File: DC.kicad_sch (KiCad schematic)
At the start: 39 parts, among them U6 MCP2551-I-P, U7 NUCLEO-F302R8

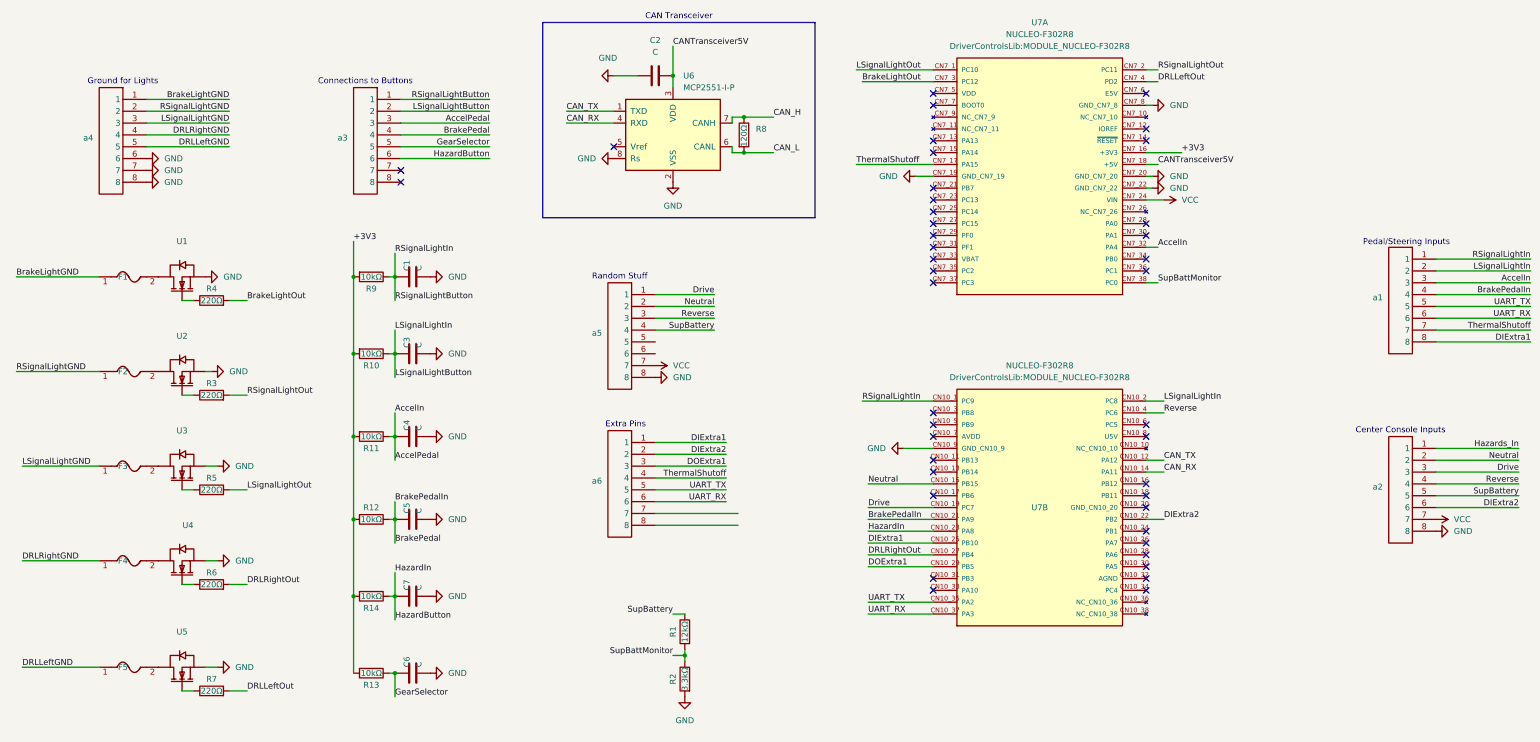
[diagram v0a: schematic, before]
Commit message: almost final draft
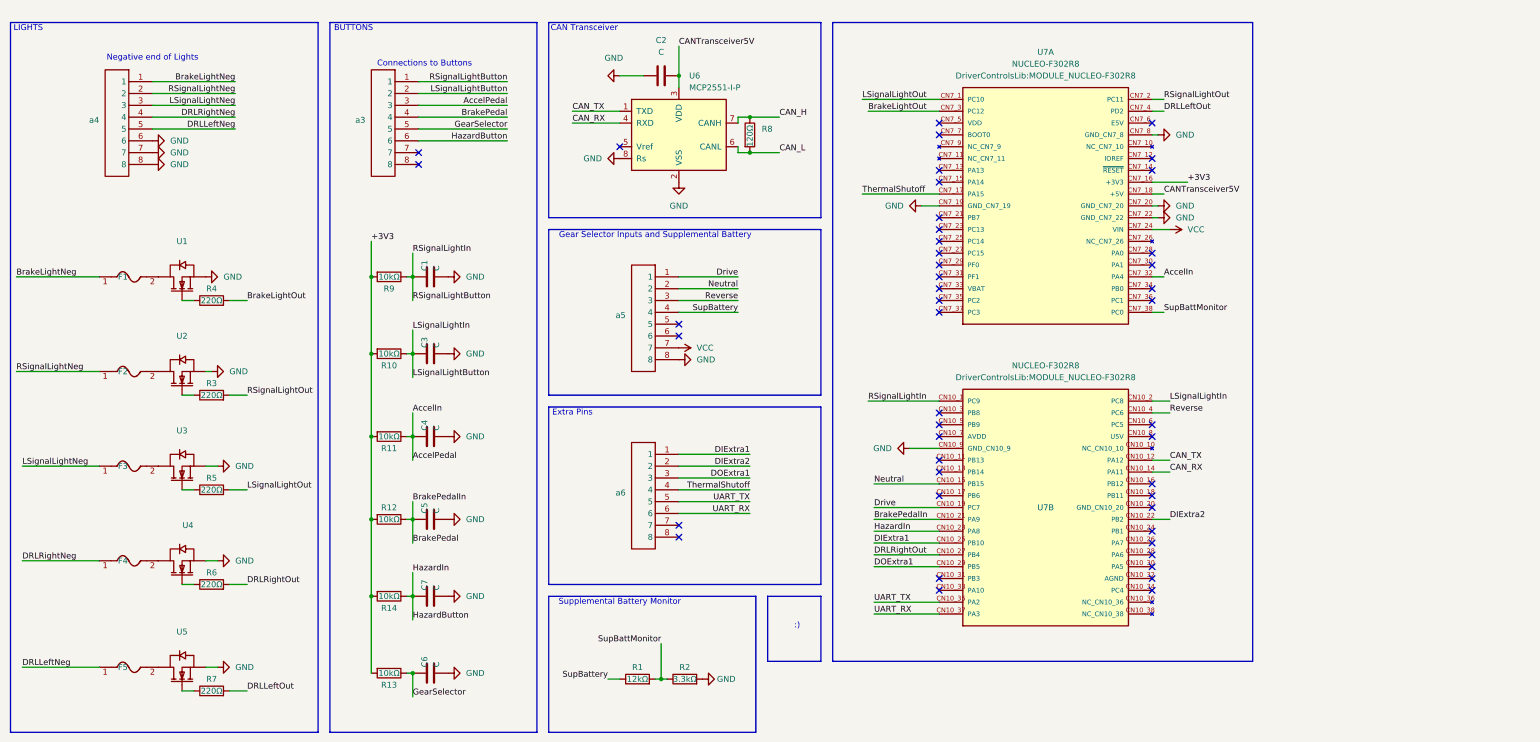
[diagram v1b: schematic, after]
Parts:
- removed a1, a2: ~, DriverControlsLib:Molex 8 Pin Mini-fit TPA, symbol DriverControlsLib:8 pin connector
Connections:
- net BrakeLightGND renamed BrakeLightNeg
- net DRLLeftGND renamed DRLLeftNeg
- net DRLRightGND renamed DRLRightNeg
- net LSignalLightGND renamed LSignalLightNeg
- net RSignalLightGND renamed RSignalLightNeg
- no-connect marks 42 -> 46
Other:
- note added: ":)"
- note added: "BUTTONS"
- note added: "Gear Selector Inputs and Supplemental Battery"
- note added: "LIGHTS"
- note added: "Negative end of Lights"
- note added: "Supplemental Battery Monitor"
- note removed: "Center Console Inputs"
- note removed: "Ground for Lights"
- note removed: "Pedal/Steering Inputs"
- note removed: "Random Stuff"
- moved on the sheet: C1, C2, C3, C4, C5, C6, C7, R1, R10, R11, R12, R13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
